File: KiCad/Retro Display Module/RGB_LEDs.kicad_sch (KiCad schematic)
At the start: 25 parts, among them J21 Conn_01x02_Pin, J23 Conn_01x02_Pin, J24 Conn_01x04_Pin, J25 Conn_02x03_Odd_Even, U4 2N7002

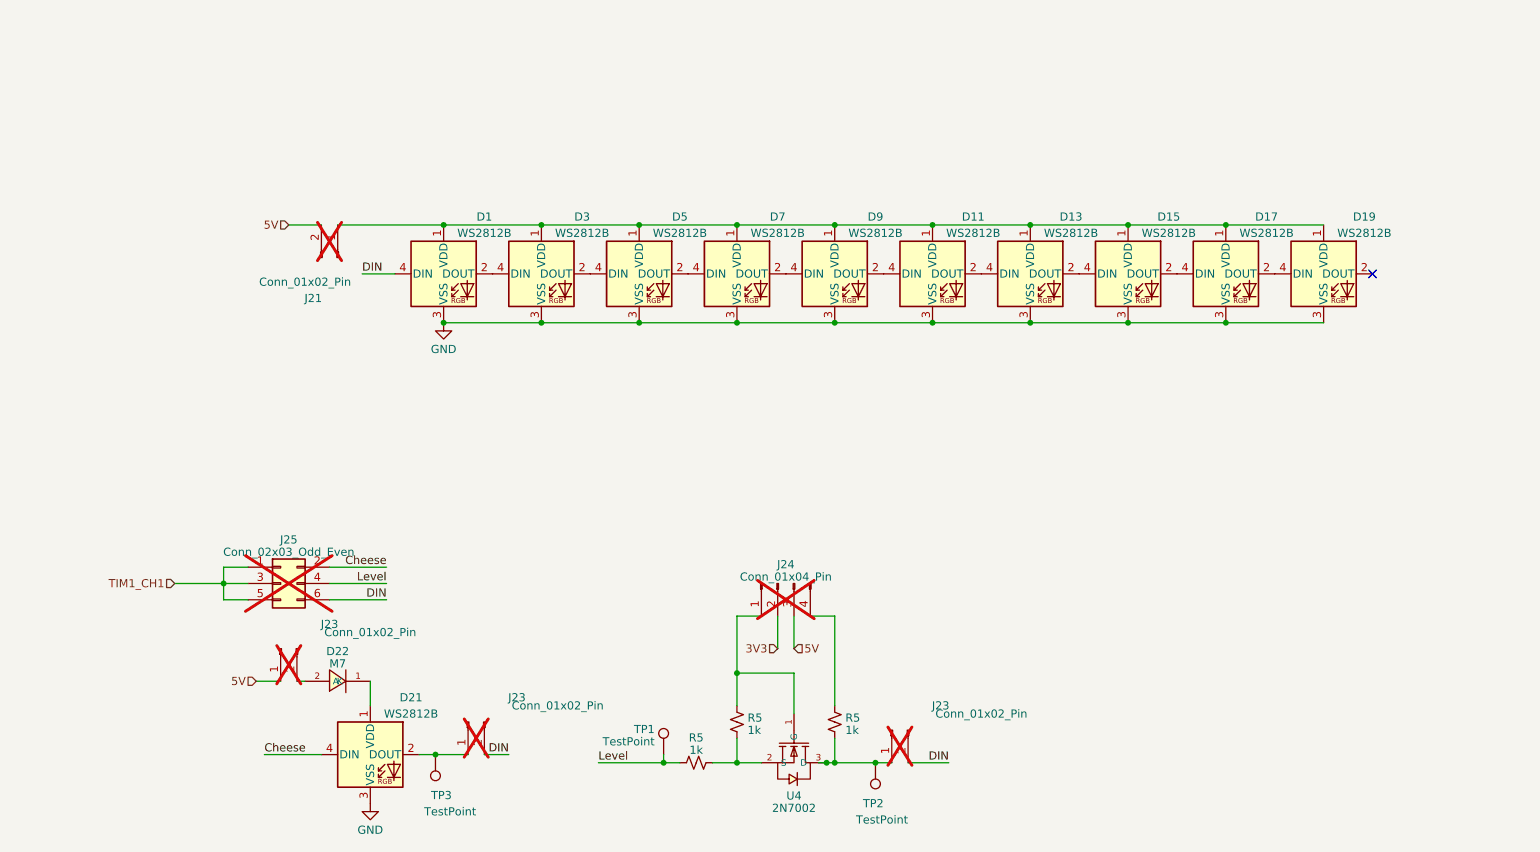
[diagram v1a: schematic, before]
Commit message: Begin STM32 Programming
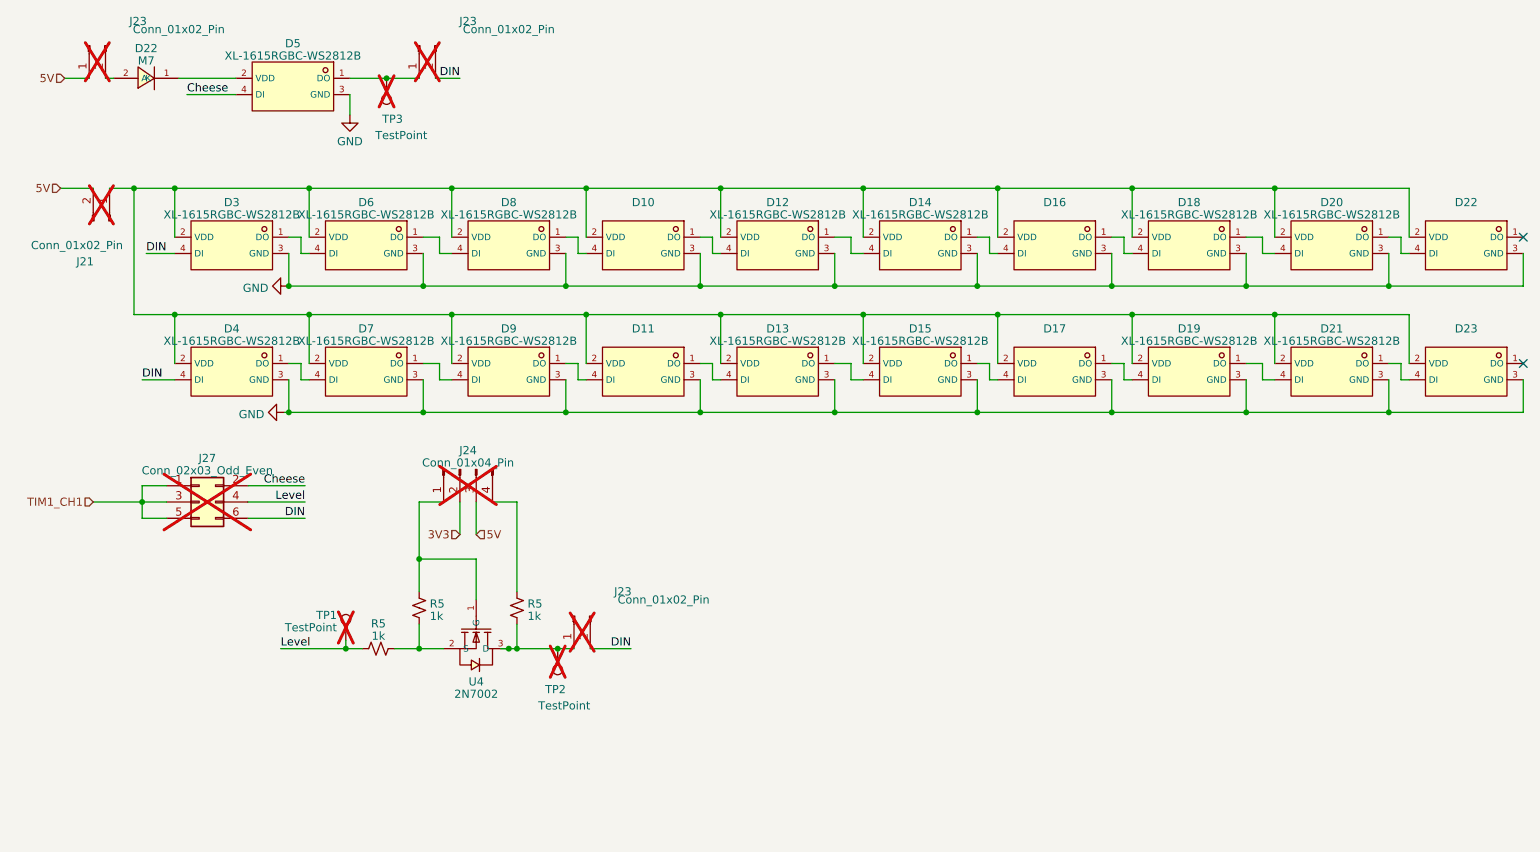
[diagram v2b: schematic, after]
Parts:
- removed D1, D11, D13, D15, D17, D19, D21, D3, D5, D7, D9: WS2812B, Library:LED-SMD_4P-L5.0-W5.0-BL_XL-5050RGBC, symbol LED:WS2812B
- added D10, D11, D12, D13, D14, D15, D16, D17, D18, D19, D20, D21, D22, D23, D3, D4, D5, D6, D7, D8, D9: XL-1615RGBC-WS2812B, Library:LED-SMD_4P-L1.6-W1.5_XL-1615RGBC-WS2812B, symbol EEE4022S:XL-1615RGBC-WS2812B
- J21, J23, J24: now left out of the parts list
- TP1, TP2, TP3: now not fitted; now left out of the parts list
- renumbered J25 to J27
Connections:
- net Cheese: now also D5.4 (DI)
- net DIN: now also D3.4 (DI), D4.4 (DI)
- net GND: now also D10.3 (GND), D11.3 (GND), D12.3 (GND), D13.3 (GND), D14.3 (GND), D15.3 (GND), D16.3 (GND), D17.3 (GND), D18.3 (GND), D19.3 (GND), D20.3 (GND), D21.3 (GND), D22.3 (GND), D23.3 (GND), D3.3 (GND), D4.3 (GND), D5.3 (GND), D6.3 (GND), D7.3 (GND), D8.3 (GND), D9.3 (GND)
- net at J21.1 (Pin_1): now also D10.2 (VDD), D11.2 (VDD), D12.2 (VDD), D13.2 (VDD), D14.2 (VDD), D15.2 (VDD), D16.2 (VDD), D17.2 (VDD), D18.2 (VDD), D19.2 (VDD), D20.2 (VDD), D21.2 (VDD), D22.2 (VDD), D23.2 (VDD), D3.2 (VDD), D4.2 (VDD), D6.2 (VDD), D7.2 (VDD), D8.2 (VDD), D9.2 (VDD)
- net at J23.1 (Pin_1), TP3.1: now also D5.1 (DO)
- net at D22.1 (K): now also D5.2 (VDD)
- new net: D12.1 (DO), D14.4 (DI)
- new net: D10.1 (DO), D12.4 (DI)
- new net: D13.1 (DO), D15.4 (DI)
- new net: D11.1 (DO), D13.4 (DI)
- new net: D16.1 (DO), D18.4 (DI)
- new net: D14.1 (DO), D16.4 (DI)
- new net: D19.1 (DO), D21.4 (DI)
- new net: D17.1 (DO), D19.4 (DI)
- new net: D7.1 (DO), D9.4 (DI)
- new net: D4.1 (DO), D7.4 (DI)
- new net: D6.1 (DO), D8.4 (DI)
- new net: D3.1 (DO), D6.4 (DI)
- new net: D15.1 (DO), D17.4 (DI)
- new net: D10.4 (DI), D8.1 (DO)
- new net: D20.1 (DO), D22.4 (DI)
- new net: D18.1 (DO), D20.4 (DI)
- new net: D11.4 (DI), D9.1 (DO)
- new net: D21.1 (DO), D23.4 (DI)
- no-connect marks 1 -> 2
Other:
- moved on the sheet: D22, J21, J23, J24, J27, R5, U4
